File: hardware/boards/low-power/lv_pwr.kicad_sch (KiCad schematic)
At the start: 20 parts, among them U13 INA2180A3IDSGR

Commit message: Add footprints and models for LP board
Also completed rough layout for LP board to estimate board space usage.
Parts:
- L? (x2): footprint capstone:MHCB06030 -> capstone:IND_LQH5BPN6R8NT0L
- U13: footprint (none) -> capstone:SON50P200X200X80-9N
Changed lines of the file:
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@@
       (effects (font (size 1.27 1.27)))
     )
-    (property "Footprint" "capstone:MHCB06030" (at 120.65 130.175 0)
+    (property "Footprint" "capstone:IND_LQH5BPN6R8NT0L" (at 120.65 130.175 0)
       (effects (font (size 1.27 1.27)) hide)
     )
@@
       (effects (font (size 1.27 1.27)))
     )
-    (property "Footprint" "capstone:MHCB06030" (at 120.015 75.565 0)
+    (property "Footprint" "capstone:IND_LQH5BPN6R8NT0L" (at 120.015 75.565 0)
       (effects (font (size 1.27 1.27)) hide)
     )
@@
       (effects (font (size 1.27 1.27)) (justify left))
     )
-    (property "Footprint" "" (at 212.09 106.045 0)
-      (effects (font (size 1.27 1.27)) hide)
-    )
+    (property "Footprint" "capstone:SON50P200X200X80-9N" (at 212.09 106.045 0)
+      (effects (font (size 1.27 1.27)) hide)
+    )

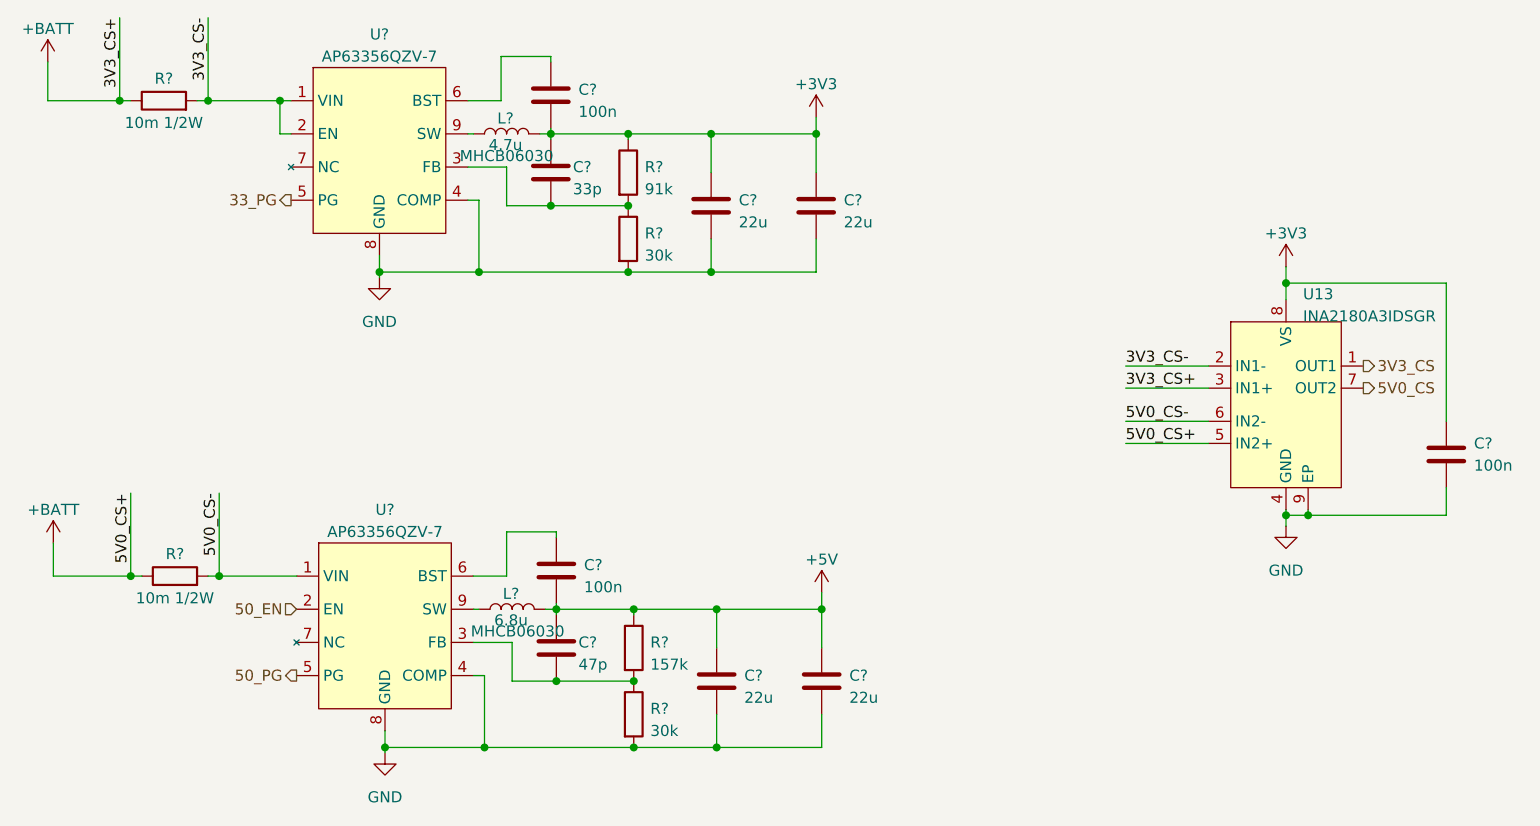
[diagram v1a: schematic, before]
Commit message: Add initial changes after schematic review
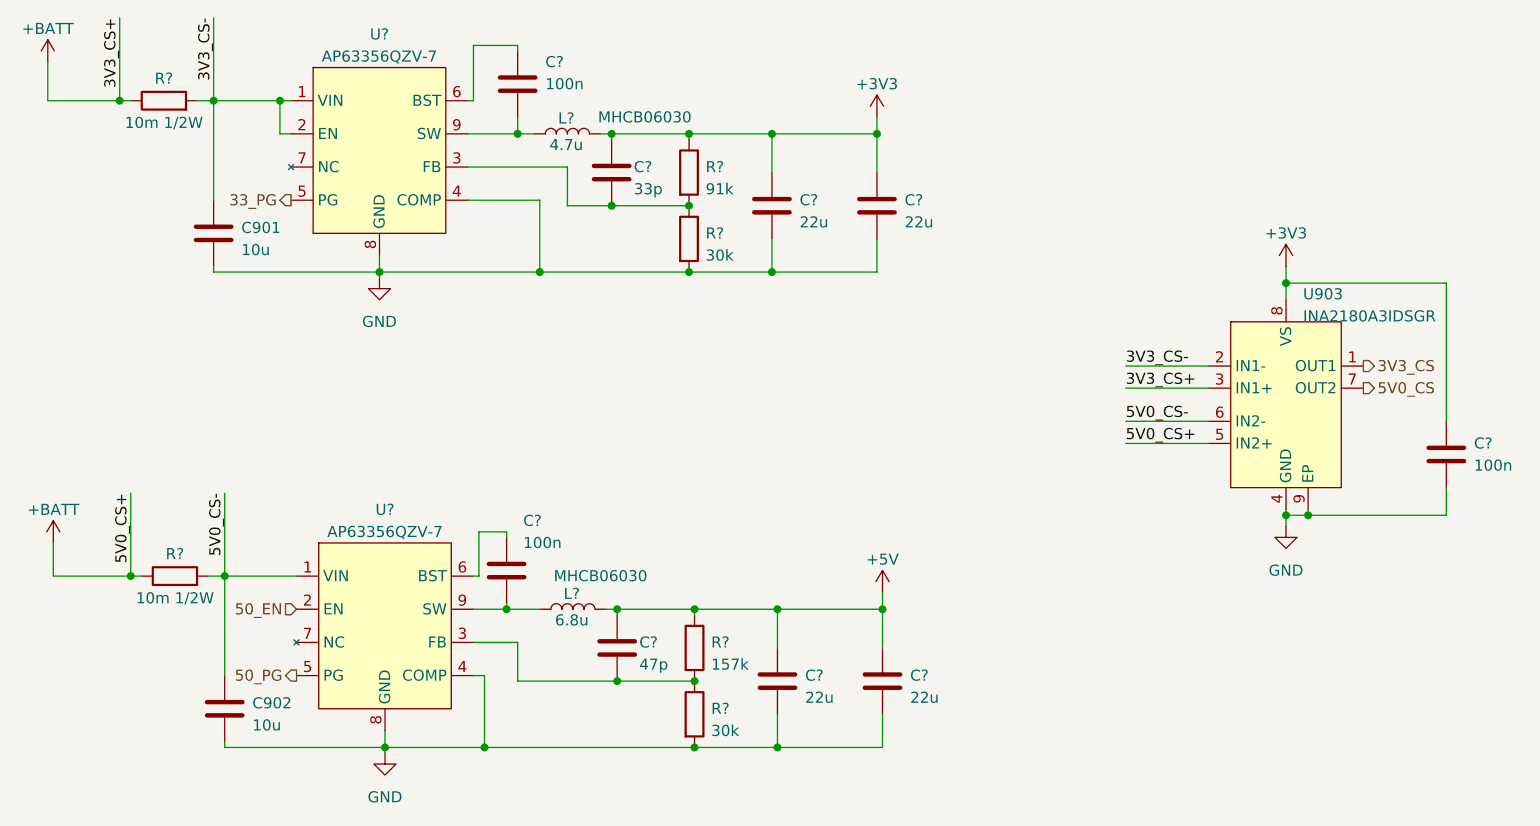
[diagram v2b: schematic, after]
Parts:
- removed C?: 100n, Capacitor_SMD:C_0201_0603Metric, symbol Device:C
- added C901, C902: 10u, symbol Device:C
- added C?: 100n, Capacitor_SMD:C_0201_0603Metric, symbol Device:C
- renumbered U13 to U903
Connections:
- net +3V3: no longer C?.2
- net 3V3_CS-: now also C901.1
- net 5V0_CS-: now also C902.1
- net GND: now also C901.2, C902.2
- net at L?.1, U?.9 (SW): now also C?.2 (x2)
- net at U?.6 (BST): now also C?.1
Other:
- moved on the sheet: C?, L?, R?
